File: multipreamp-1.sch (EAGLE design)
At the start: 116 parts, among them Q1 J201, Q2 J201, Q3 J201, Q4 J201, Q5 2N5088, Q6 J201, Q7 J201, Q8 J201

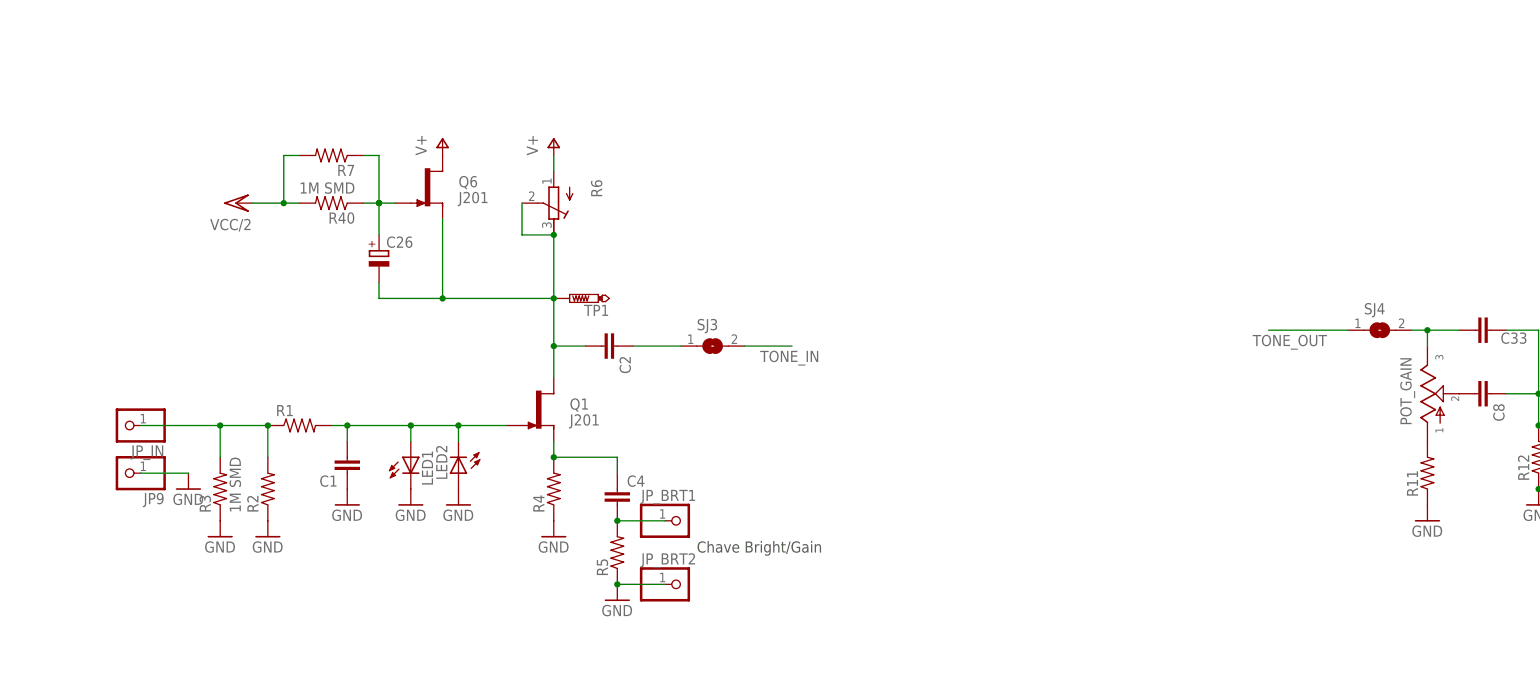
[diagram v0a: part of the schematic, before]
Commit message: Revisao do esquematico
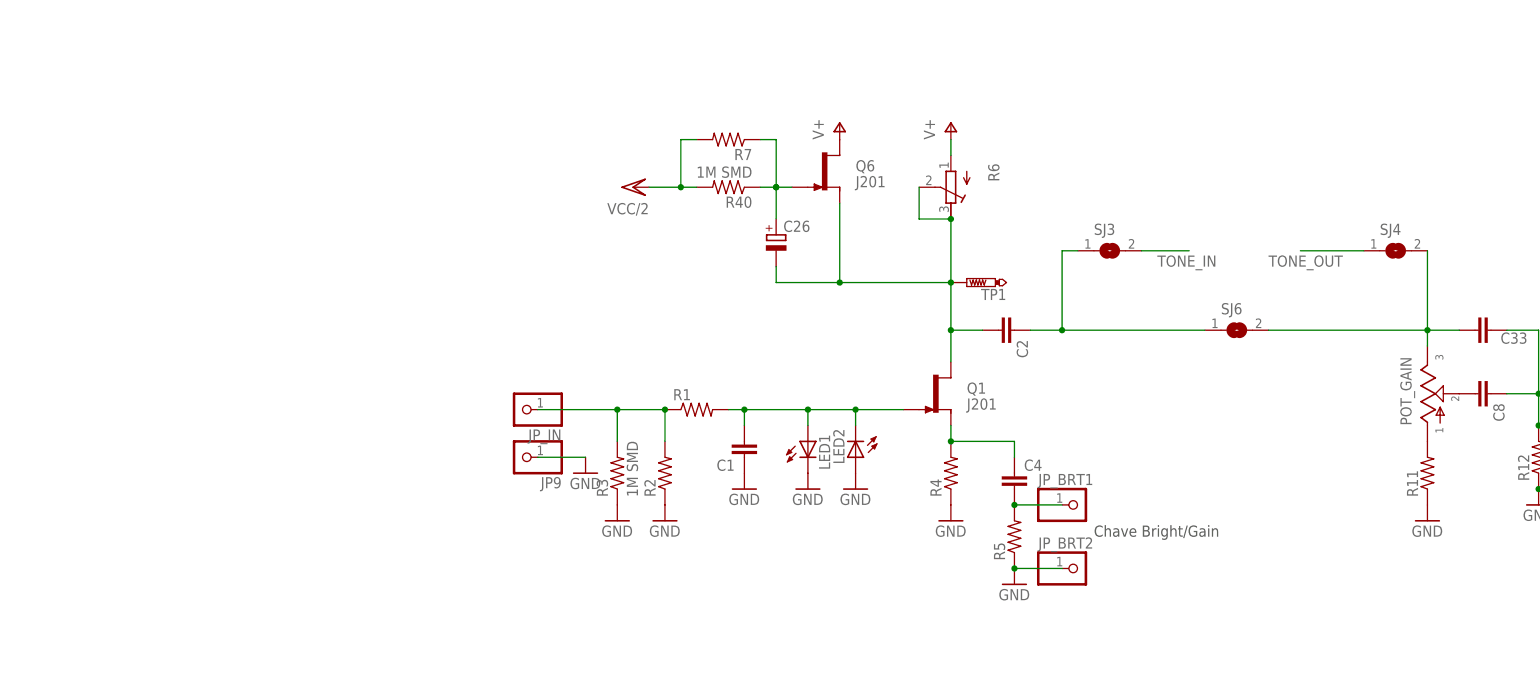
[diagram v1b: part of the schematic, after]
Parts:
- added SJ6: (no value), jumper:SJ
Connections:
- net N$11: now also SJ6.2
- net N$6: now also SJ6.1
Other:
- moved on the sheet: C1, C2, C26, C4, JP9, JP_BRT1, JP_BRT2, JP_IN, LED1, LED2, Q1, Q6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
